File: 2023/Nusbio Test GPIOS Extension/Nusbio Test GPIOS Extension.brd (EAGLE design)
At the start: 44 x 50 mm, 7 parts

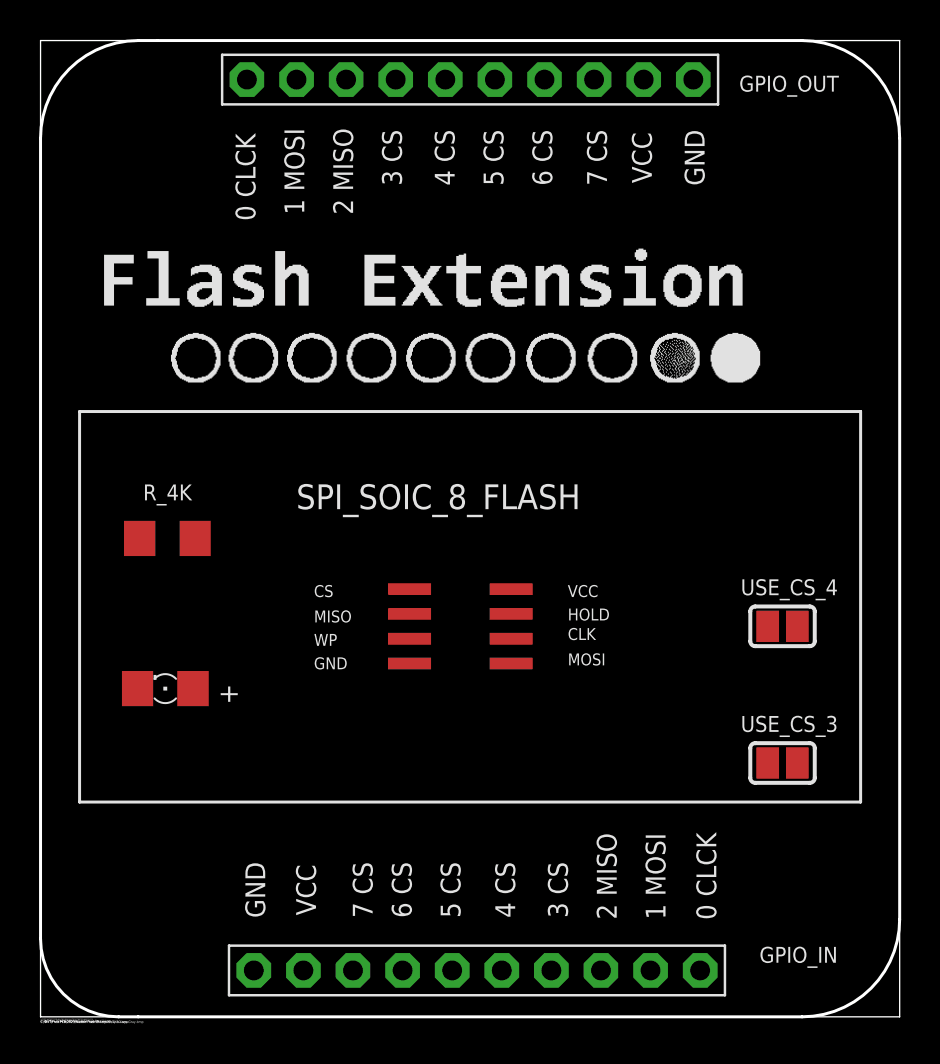
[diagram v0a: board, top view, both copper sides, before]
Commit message: Test Esxtension
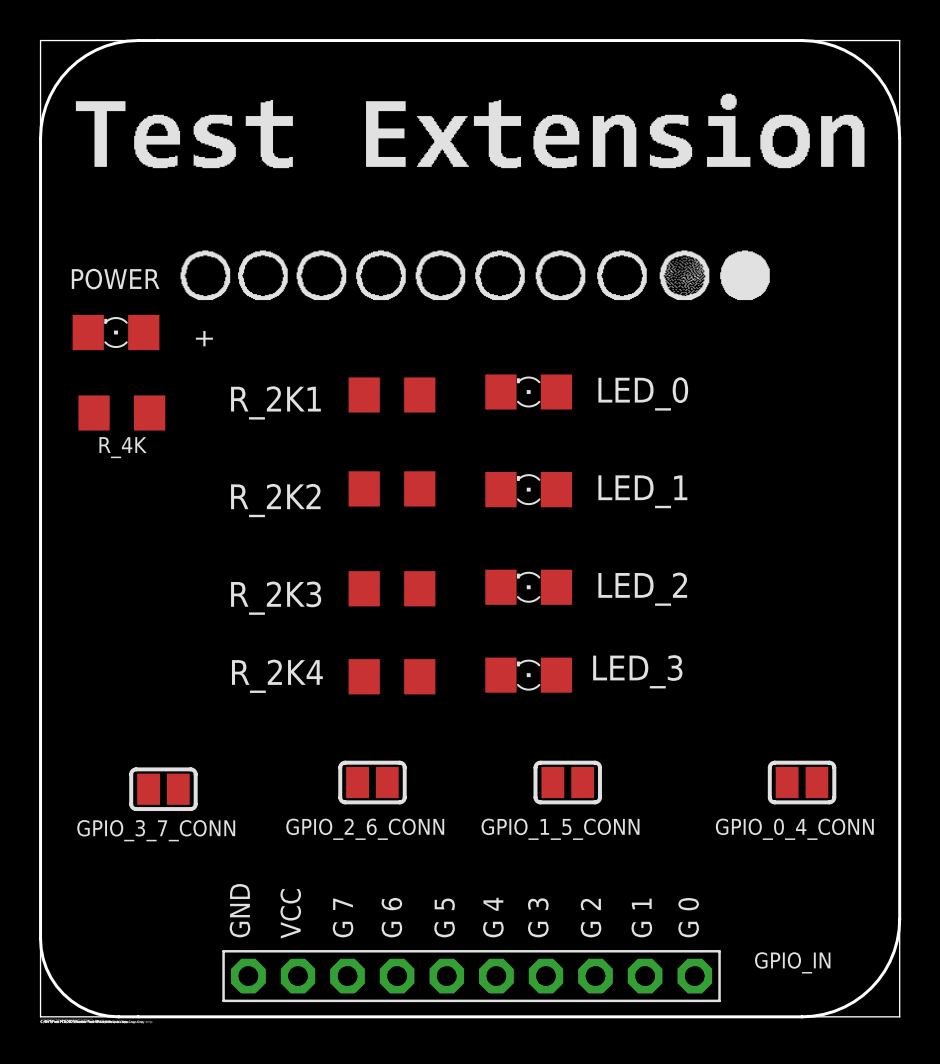
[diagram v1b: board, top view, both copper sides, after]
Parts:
- removed GPIO_OUT: PINHD-1X10, adafruit:1X10-BIG
- removed SPI_SOIC_8_FLASH: 25AA080SN, microchip:SO-08
- removed USE_CS_3, USE_CS_4: (no value), microbuilder:SOLDERJUMPER_REFLOW
- added GPIO_0_4_CONN, GPIO_1_5_CONN, GPIO_2_6_CONN, GPIO_3_7_CONN: (no value), microbuilder:SOLDERJUMPER_REFLOW
- added LED_0, LED_1, LED_2, LED_3: (no value), adafruit:1206
- added R_2K1, R_2K2, R_2K3, R_2K4: (no value), adafruit:R1206
- moved LED_POWER 18.4 mm to (3.87, 35.0)
- moved R_4K 6.84 mm to (4.17, 30.9)
- moved GPIO_IN 0.40 mm to (22.1, 2.09)
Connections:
- removed net CS: SPI_SOIC_8_FLASH.1, USE_CS_3.2, USE_CS_4.2
- removed net CS_3: GPIO_IN.4, GPIO_OUT.4, USE_CS_3.1
- removed net CS_4: GPIO_IN.5, GPIO_OUT.5, USE_CS_4.1
- removed net GPIO8: GPIO_IN.8, GPIO_OUT.8
- removed net MISO: GPIO_IN.3, GPIO_OUT.3, SPI_SOIC_8_FLASH.2
- removed net MOSI: GPIO_IN.2, GPIO_OUT.2, SPI_SOIC_8_FLASH.5
- removed net SCK: GPIO_IN.1, GPIO_OUT.1, SPI_SOIC_8_FLASH.6
- new net GPIO0: GPIO_0_4_CONN.1, GPIO_IN.1, LED_0.A
- new net GPIO1: GPIO_1_5_CONN.1, GPIO_IN.2, LED_1.A
- new net GPIO2: GPIO_2_6_CONN.1, GPIO_IN.3, LED_2.A
- new net GPIO3: GPIO_3_7_CONN.1, GPIO_IN.4, LED_3.A
- new net GPIO4: GPIO_0_4_CONN.2, GPIO_IN.5
- new net GPIO5: GPIO_1_5_CONN.2, GPIO_IN.6
- new net N$1: LED_0.C, R_2K1.2
- new net N$3: LED_1.C, R_2K2.2
- new net N$4: LED_2.C, R_2K3.2
- new net N$5: LED_3.C, R_2K4.2
- net GND: now also R_2K1.1, R_2K2.1, R_2K3.1, R_2K4.1; no longer GPIO_OUT.10, SPI_SOIC_8_FLASH.4
- net GPIO6: now also GPIO_2_6_CONN.2, GPIO_IN.7; no longer GPIO_IN.6, GPIO_OUT.6
- net GPIO7: now also GPIO_3_7_CONN.2, GPIO_IN.8; no longer GPIO_IN.7, GPIO_OUT.7
- net VCC: no longer GPIO_OUT.9, SPI_SOIC_8_FLASH.3, SPI_SOIC_8_FLASH.7, SPI_SOIC_8_FLASH.8
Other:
- board text added: "C:/DVT/Fred.PCB/2023/Nusbio Test GPIOS Extension/Title.Logo.Gray.bmp"
- board text added: "G 0"
- board text added: "G 1"
- board text added: "G 2"
- board text added: "G 3"
- board text added: "G 4"
- board text added: "G 5"
- board text added: "G 6"
- board text added: "G 7"
- board text added: "PCBv2 - 2023.04"
- board text added: "POWER"
- board text removed: "0 CLCK"
- board text removed: "1 MOSI"
- board text removed: "2 MISO"
- board text removed: "3 CS"
- board text removed: "4 CS"
- board text removed: "5 CS"
- board text removed: "6 CS"
- board text removed: "7 CS"
- board text removed: "CLK"
- board text removed: "CS"
- board text removed: "HOLD"
- board text removed: "MISO"
- board text removed: "MOSI"
- board text removed: "PCBv2 - 2023.03"
- board text removed: "WP"

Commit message: Test Esxtension
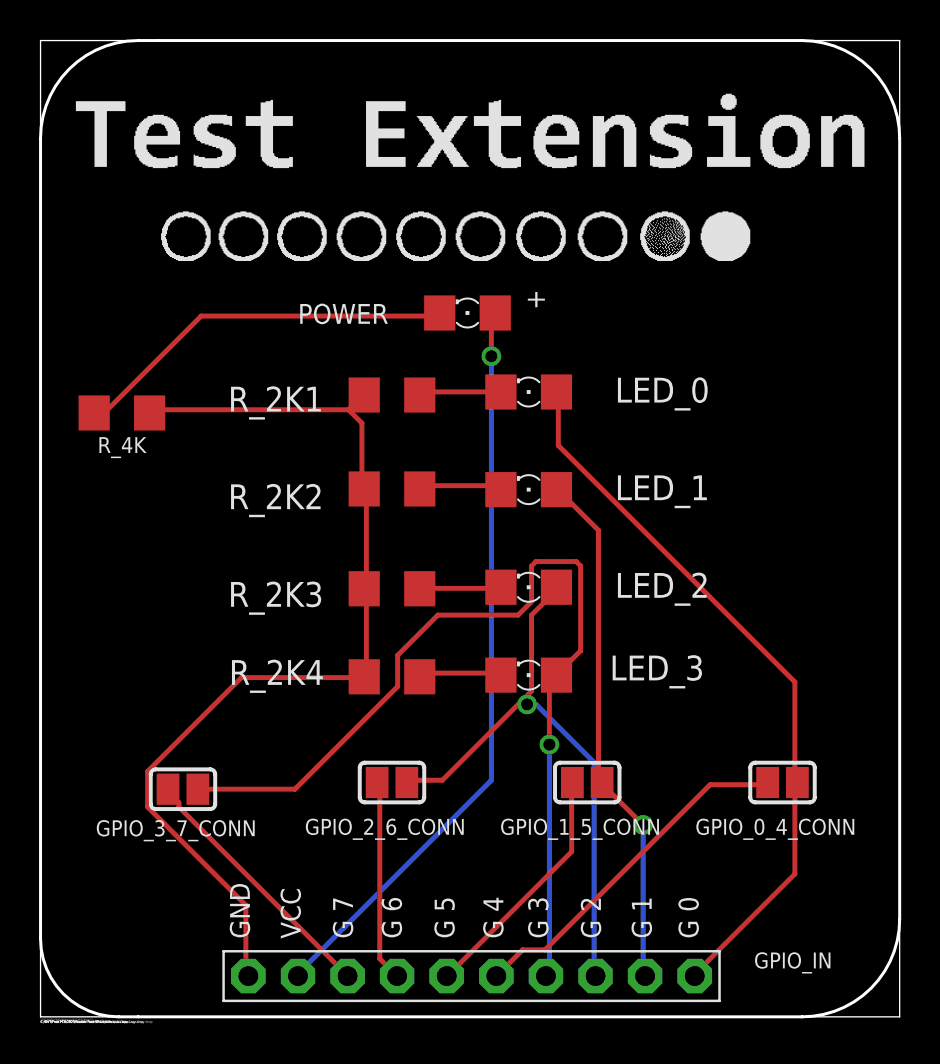
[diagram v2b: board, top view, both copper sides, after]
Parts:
- moved LED_POWER 18.0 mm to (21.9, 36.0)
- moved GPIO_0_4_CONN 1.00 mm to (38.0, 12.0)
- moved GPIO_1_5_CONN 1.00 mm to (28.0, 12.0)
- moved GPIO_2_6_CONN 1.00 mm to (18.0, 12.0)
- moved GPIO_3_7_CONN 1.00 mm to (7.29, 11.7)
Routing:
- net GND: track 0.00 -> 51.3 mm
- net GPIO3: track 0.00 -> 48.3 mm, vias 0 -> 1
- net VCC: track 0.00 -> 38.1 mm, vias 0 -> 1
- net GPIO0: track 0.00 -> 37.2 mm
- net GPIO2: track 0.00 -> 30.2 mm, vias 0 -> 1
- net GPIO1: track 0.00 -> 26.8 mm, vias 0 -> 1
- net N$2: track 0.00 -> 19.8 mm
- net GPIO4: track 0.00 -> 18.0 mm
- net GPIO7: track 0.00 -> 13.4 mm
- net GPIO5: track 0.00 -> 12.6 mm
- net GPIO6: track 0.00 -> 10.3 mm
- net N$3: track 0.00 -> 4.49 mm
- net N$5: track 0.00 -> 4.41 mm
- net N$1: track 0.00 -> 4.31 mm
- net N$4: track 0.00 -> 4.20 mm
